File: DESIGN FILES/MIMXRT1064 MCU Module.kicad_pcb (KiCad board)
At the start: 2 copper layers, 99.1 x 66 mm, 102 parts, among them J601 TF-15x15, Q601 IRLML6401, U1 MIMXRT1064CVL5B, U301 UM805RE, U302 UM803RS, U601 IS42S16160J-6BLI, U602 IS25WP064A-JBLE, Y401 7V24000026, Y402 X201232768KJD2SI

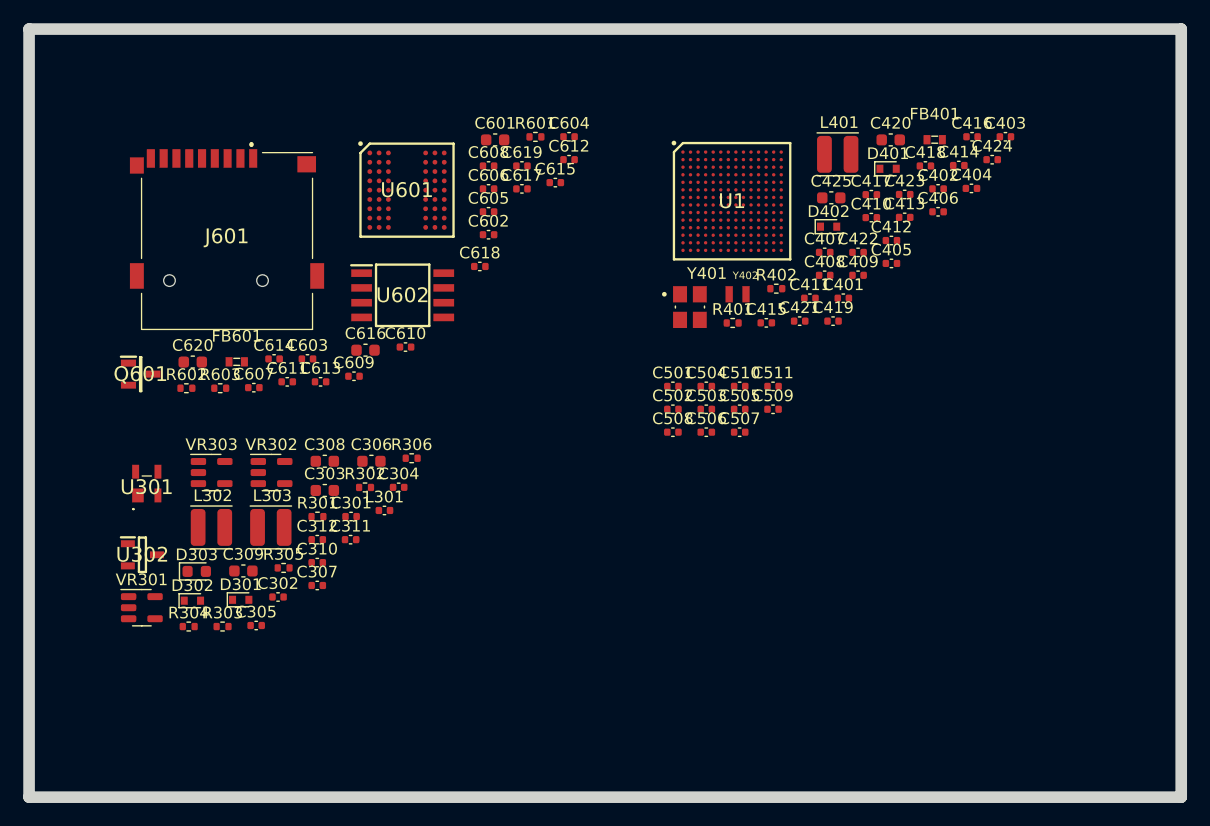
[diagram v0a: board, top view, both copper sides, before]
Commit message: schematic changes
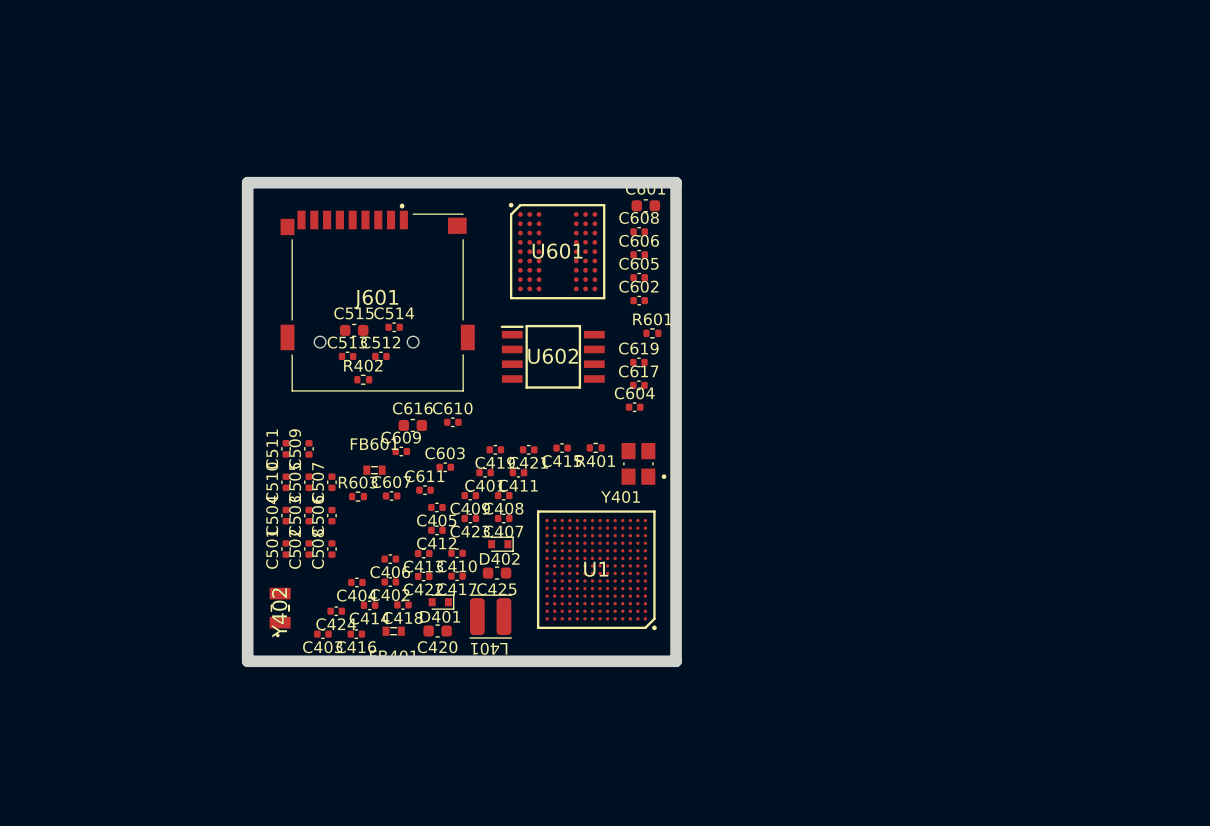
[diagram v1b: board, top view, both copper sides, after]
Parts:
- removed C301, C302, C310, C612, C614: 1u, MIMXRT1064 MCU Module:0402_CL05A105KA5NQNC
- removed C303, C308: 22u, MIMXRT1064 MCU Module:0603_CL10A226MQ8NRNC
- removed C304, C305, C307, C618: 100n, MIMXRT1064 MCU Module:0402_CL05B104KB54PNC
- removed C306, C309, C620: 10u, MIMXRT1064 MCU Module:0603_CL10A106KP8NNNC
- removed C311, L301: 10n, MIMXRT1064 MCU Module:0402_CL05B103KB5NNNC
- removed C312: 10u, MIMXRT1064 MCU Module:0402_CL05B103KB5NNNC
- removed C613, C615: 1uF, MIMXRT1064 MCU Module:0402_CL05A105KA5NQNC
- removed D301, D302: RB521S30_R1_00001, MIMXRT1064 MCU Module:RB521S30_R1_00001
- removed D303: ~, MIMXRT1064 MCU Module:19-218_BHC-ZL1M2QY_3T
- removed L302, L303: 2.2u, MIMXRT1064 MCU Module:CD32YP0302-2R2M_SMD3.5x3x2.1mm
- removed Q601: IRLML6401, MIMXRT1064 MCU Module:IRLML6401
- removed R301, R602: 10k, MIMXRT1064 MCU Module:0402WGF1002TCE
- removed R302, R306: 100k, MIMXRT1064 MCU Module:0402WGF1003TCE
- removed R303: 22k, MIMXRT1064 MCU Module:0402WGF2202TCE
- removed R304: 2.2k, MIMXRT1064 MCU Module:0402WGF2201TCE
- removed R305: 200k, MIMXRT1064 MCU Module:0402WGF2003TCE
- removed U301: UM805RE, MIMXRT1064 MCU Module:UM805RE
- removed U302: UM803RS, MIMXRT1064 MCU Module:UM803RS
- removed VR301, VR302: TLV62569DBV, MIMXRT1064 MCU Module:TLV62569DBVR
- removed VR303: TPS79333DBVR, MIMXRT1064 MCU Module:TPS79333DBVR_SOT-23-5
- added C512: 1u, MIMXRT1064 MCU Module:0402_CL05A105KA5NQNC, F.Cu at (162.3, 78.9)
- added C513: 1u, MIMXRT1064 MCU Module:0402_CL05A105KA5NQNC, F.Cu at (159.5, 78.9)
- added C514: 100n, MIMXRT1064 MCU Module:0402_CL05B104KB54PNC, F.Cu at (163.5, 76.4)
- added C515: 10u, MIMXRT1064 MCU Module:0603_CL10A106KP8NNNC, F.Cu at (160.0, 76.7)
- R402: footprint MIMXRT1064 MCU Module:0402WGF3302TCE -> MIMXRT1064 MCU Module:AF0402FR-0730KL
- Y402: value X201232768KJD2SI -> Q13FC1350000200; footprint MIMXRT1064 MCU Module:X201232768KJD2SI -> MIMXRT1064 MCU Module:Q13FC1350000200
- moved C403 72.6 mm to (157.3, 102.8), turned to 180 degrees
- moved C424 68.5 mm to (158.5, 100.9), turned to 180 degrees
- moved C416 68.1 mm to (160.2, 102.8), turned to 180 degrees
- moved C414 63.2 mm to (161.4, 100.4), turned to 180 degrees
- moved FB401 62.8 mm to (163.4, 102.6), turned to 180 degrees
- moved C404 62.8 mm to (160.3, 98.4), turned to 180 degrees
- moved C418 58.7 mm to (164.2, 100.3), turned to 180 degrees
- moved C402 58.0 mm to (163.1, 98.3), turned to 180 degrees
- moved C420 57.4 mm to (167.2, 102.6), turned to 180 degrees
- moved C406 55.8 mm to (163.1, 96.4), turned to 180 degrees
- moved D401 53.6 mm to (167.4, 100.1), turned to 180 degrees
- moved C422 52.8 mm to (166.0, 97.9), turned to 180 degrees
- moved C413 50.5 mm to (166.0, 95.9), turned to 180 degrees
- moved C417 48.4 mm to (168.9, 97.8), turned to 180 degrees
- moved Y402 47.7 mm to (153.7, 100.6), turned to 90 degrees
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- renumbered C423 to C422, C422 to C423
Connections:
- net USB_OTG1_DN renamed USB_OTG1_D-
- net USB_OTG1_DP renamed USB_OTG1_D+
- net USB_OTG2_DN renamed USB_OTG2_D-
- net USB_OTG2_DP renamed USB_OTG2_D+
- R402 pad 1: /MCU POWER & CRYSTALS/DCDC_PSWITCH -> /MCU POWER & CRYSTALS/DCDC_IN
- R402 pad 2: /MCU POWER & CRYSTALS/DCDC_IN -> /MCU POWER & CRYSTALS/DCDC_PSWITCH
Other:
- board size 99.1 x 66 mm -> 36.8 x 41.1 mm
